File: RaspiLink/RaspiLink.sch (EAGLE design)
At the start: 20 parts, among them Q1 MOSFET-NCHANNELBSS123LT1G, Q2 MOSFET-NCHANNELBSS123LT1G, X1 SSW-120-02-S-D, X2 SSW-120-02-S-S, X3 SSW-120-02-S-S, X4 SSW-108-02-S-D

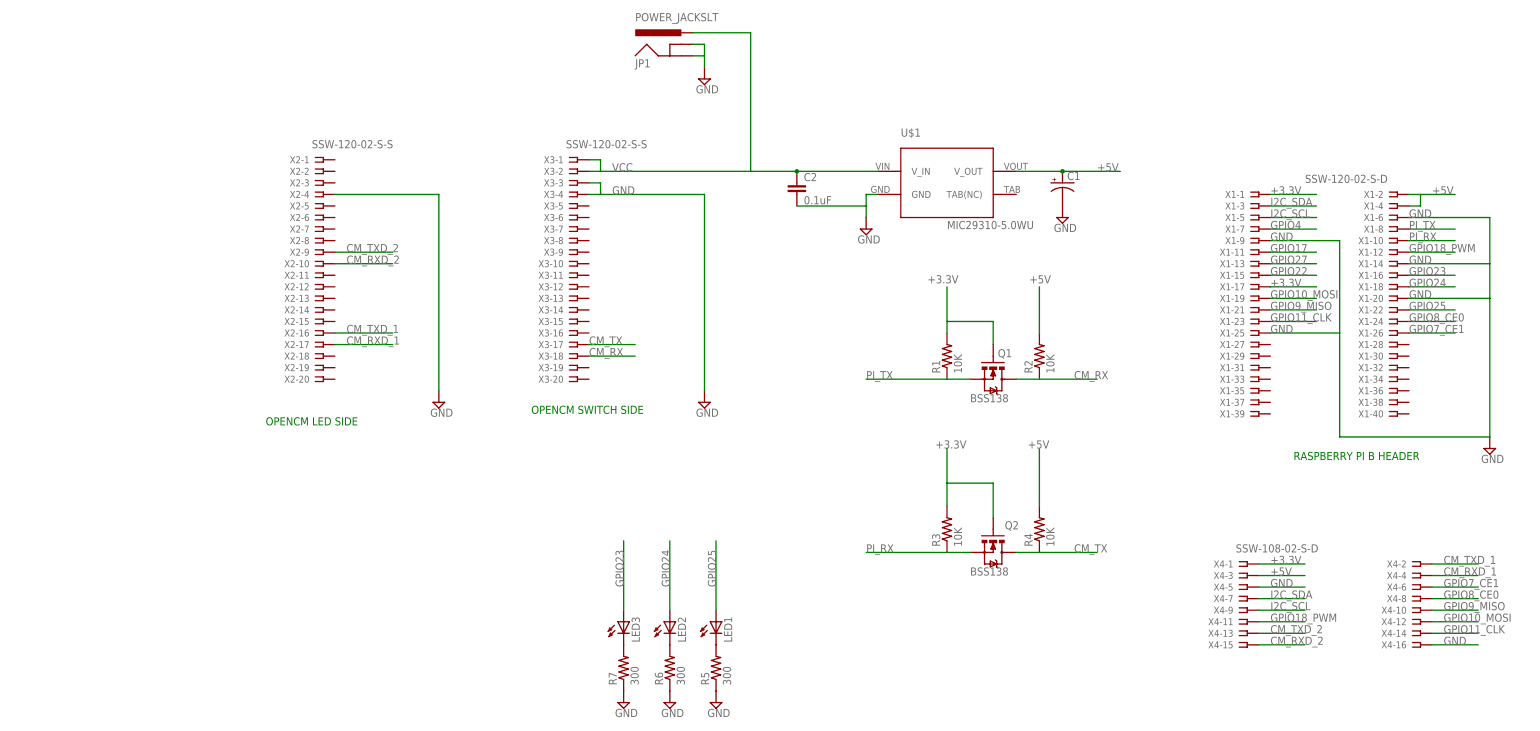
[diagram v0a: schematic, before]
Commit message: joystick for crane
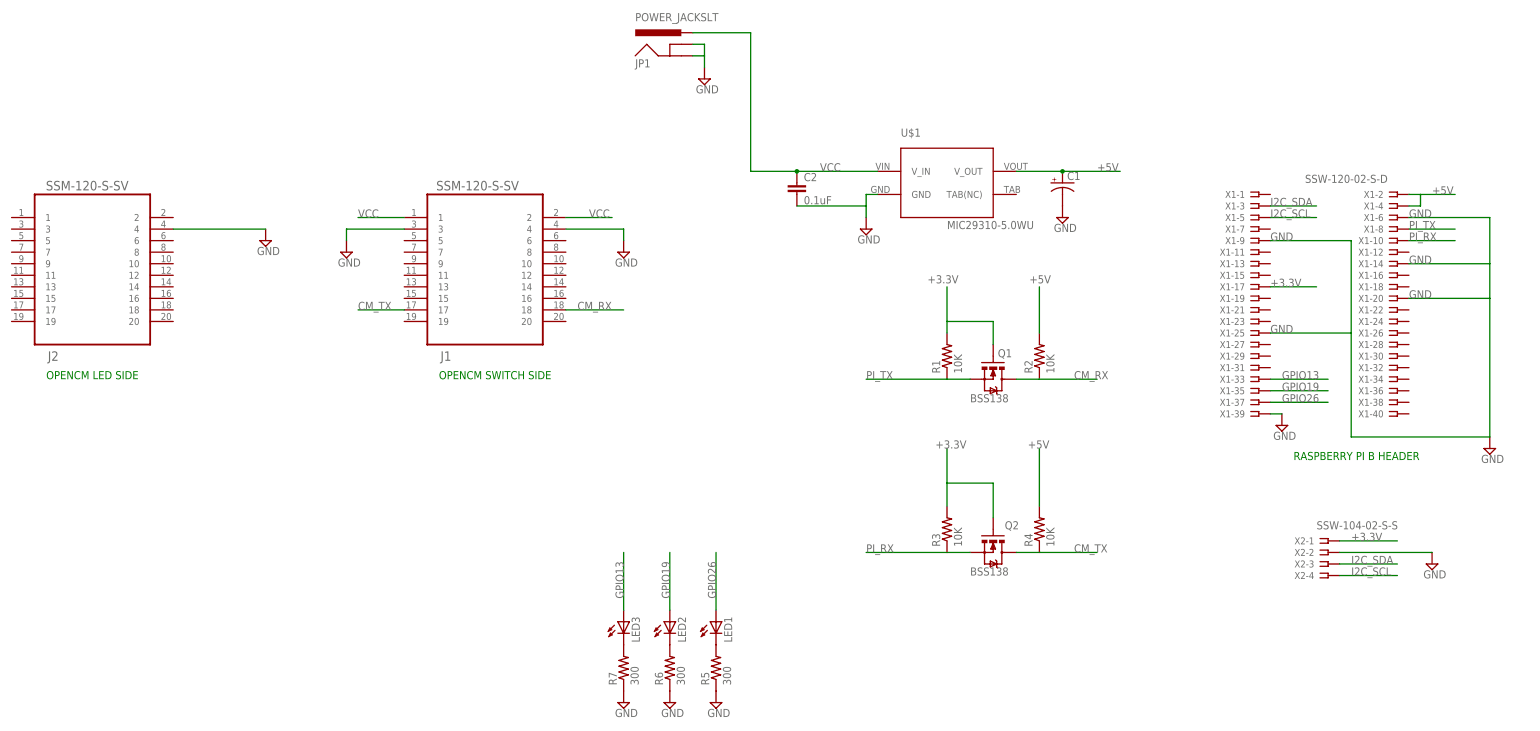
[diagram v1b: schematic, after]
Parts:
- removed X3: SSW-120-02-S-S, con-samtec:SSW-120-02-S-S
- removed X4: SSW-108-02-S-D, con-samtec:SSW-108-02-S-D
- added J1, J2: SSM-120-S-SV, SAMTEC-FLE-Mxx-Sxx_By_element14_Batch_1:SSM-120-S-SV
- X2: value SSW-120-02-S-S -> SSW-104-02-S-S; device con-samtec:SSW-120-02-S-S -> con-samtec:SSW-104-02-S-S
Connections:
- removed net CM_RXD_1: X2-17.1, X4-4.1
- removed net CM_RXD_2: X2-10.1, X4-15.1
- removed net CM_TXD_1: X2-16.1, X4-2.1
- removed net CM_TXD_2: X2-9.1, X4-13.1
- removed net GPIO10_MOSI: X1-19.1, X4-12.1
- removed net GPIO11_CLK: X1-23.1, X4-14.1
- removed net GPIO17: X1-11.1
- removed net GPIO18_PWM: X1-12.1, X4-11.1
- removed net GPIO22: X1-15.1
- removed net GPIO23: LED3.A, X1-16.1
- removed net GPIO24: LED2.A, X1-18.1
- removed net GPIO25: LED1.A, X1-22.1
- removed net GPIO27: X1-13.1
- removed net GPIO4: X1-7.1
- removed net GPIO7_CE1: X1-26.1, X4-6.1
- removed net GPIO8_CE0: X1-24.1, X4-8.1
- removed net GPIO9_MISO: X1-21.1, X4-10.1
- new net GPIO13: LED3.A, X1-33.1
- new net GPIO19: LED2.A, X1-35.1
- new net GPIO26: LED1.A, X1-37.1
- net +3.3V: now also X2-1.1; no longer X1-1.1, X4-1.1
- net +5V: no longer X4-3.1
- net CM_RX: now also J1.18; no longer X3-18.1
- net CM_TX: now also J1.17; no longer X3-17.1
- net GND: now also J1.3, J1.4, J2.4, X1-39.1, X2-2.1; no longer X2-4.1, X3-3.1, X3-4.1, X4-16.1, X4-5.1
- net I2C_SCL: now also X2-4.1; no longer X4-9.1
- net I2C_SDA: now also X2-3.1; no longer X4-7.1
- net VCC: now also J1.1, J1.2; no longer X3-1.1, X3-2.1
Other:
- moved on the sheet: X2-1, X2-2, X2-3, X2-4
